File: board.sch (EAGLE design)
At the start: 75 parts, among them IC1 LM1117, J1 LHBEAMOUT, J10 ATEMP, J11 HORNOUT, J12 12V_SUPPLY, J13 STOPOUT, J14 TURNOUT, J15 FANOUT, J16 BLIGHTOUT, J17 AUXOUT, J18 AUX, J19 CAN, J2 BATT, J3 BLIGHT, J4 LHBEAM, J5 LRTURN, J6 WARNING, J7 HORN, J8 BREAK, J9 ABREAK, Q1 IRF7465TR, Q2 IRF7465TR, Q3 IRF7465TR, Q4 IRLML9301TRPBF, Q5 IRLML9301TRPBF, Q6 IRF7424TRPBF, Q7 IRF7424TRPBF, Q8 IRF7424TRPBF, Q9 IRLML9301TRPBF, U1 VOM1271T, U2 VOM1271T, U3 VOM1271T, U4 MC14504BDR2G, U5 MAX3051ESA+T

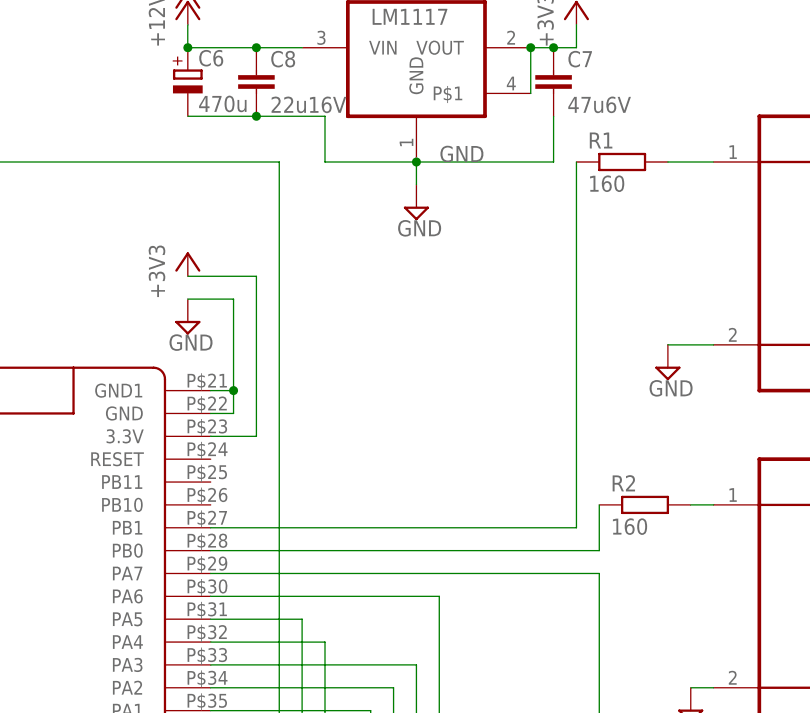
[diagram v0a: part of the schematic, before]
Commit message: Board & schematics v 1.1. Minor improvements
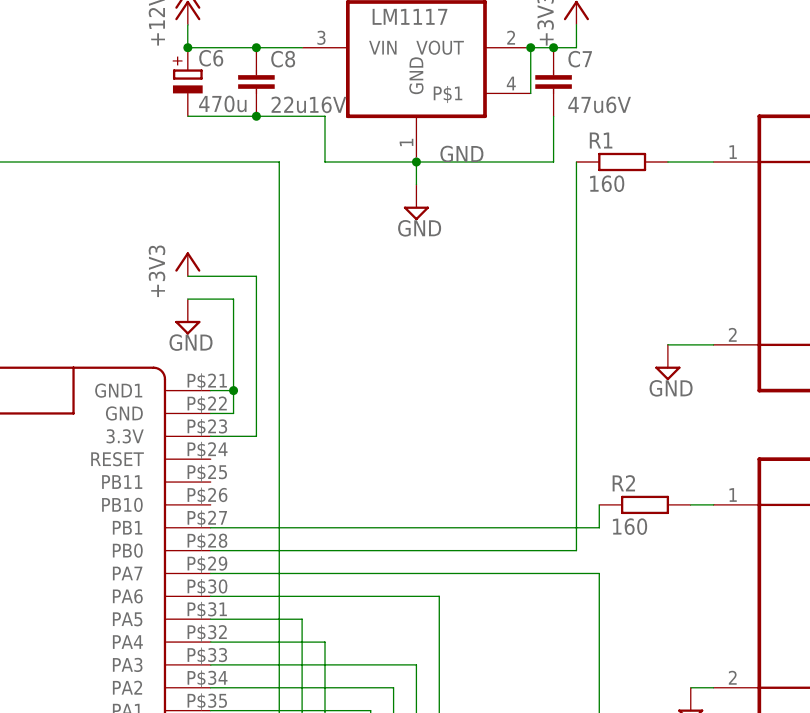
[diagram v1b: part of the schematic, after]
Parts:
- C2: device rcl:C-EUC0805 -> rcl:C-EUC1206
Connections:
- net N$1 renamed LVCTL4
- net N$13 renamed LVCTL2
- net N$14 renamed LVCTL3
- net N$2 renamed LVCTL5
- net N$20 renamed LV4G
- net N$24 renamed LV5G
- net N$25 renamed LV6G
- net N$26 renamed LV3G
- net N$27 renamed LV2G
- net N$28 renamed LV1G
- net N$3 renamed LVCTL6
- net N$37 renamed IATEMP
- net N$38 renamed ABRK
- net N$39 renamed ABRK_S
- net N$4 renamed HV1CTLG
- net N$5 renamed HV2CTLG
- net N$6 renamed HV3CTLG
- net N$7 renamed HV1G
- net N$8 renamed HV2G
- net N$9 renamed HV3G
- net HV1CTL: now also U$1.PB0; no longer U$1.PB1
- net HV2CTL: now also U$1.PB1; no longer U$1.PB0
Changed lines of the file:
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@@
 </spice>
 </part>
-<part name="C2" library="rcl" library_urn="urn:adsk.eagle:library:334" deviceset="C-EU" device="C0805" package3d_urn="urn:adsk.eagle:package:23617/2" value="0.1u"/>
+<part name="C2" library="rcl" library_urn="urn:adsk.eagle:library:334" deviceset="C-EU" device="C1206" package3d_urn="urn:adsk.eagle:package:23618/2" value="0.1u"/>
 <part name="C3" library="rcl" library_urn="urn:adsk.eagle:library:334" deviceset="C-EU" device="C0805" package3d_urn="urn:adsk.eagle:package:23617/2" value="0.1u"/>
 <part name="LOGO2" library="SparkFun-Aesthetics" deviceset="OSHW-LOGO" device="L"/>
@@
 <net name="HV1CTL" class="0">
 <segment>
+<pinref part="R1" gate="G$1" pin="1"/>
+<wire x1="-20.32" y1="114.3" x2="-20.32" y2="157.48" width="0.1524" layer="91"/>
+<pinref part="U$1" gate="G$1" pin="PB0"/>
+<wire x1="-20.32" y1="114.3" x2="-60.96" y2="114.3" width="0.1524" layer="91"/>
+</segment>
+</net>
+<net name="HV2CTL" class="0">
+<segment>
+<pinref part="R2" gate="G$1" pin="1"/>
 <pinref part="U$1" gate="G$1" pin="PB1"/>
-<wire x1="-60.96" y1="116.84" x2="-20.32" y2="116.84" width="0.1524" layer="91"/>
-<pinref part="R1" gate="G$1" pin="1"/>
-<wire x1="-20.32" y1="116.84" x2="-20.32" y2="157.48" width="0.1524" layer="91"/>
-</segment>
-</net>
-<net name="HV2CTL" class="0">
-<segment>
-<pinref part="U$1" gate="G$1" pin="PB0"/>
-<wire x1="-60.96" y1="114.3" x2="-17.78" y2="114.3" width="0.1524" layer="91"/>
-<wire x1="-17.78" y1="114.3" x2="-17.78" y2="119.38" width="0.1524" layer="91"/>
-<pinref part="R2" gate="G$1" pin="1"/>
+<wire x1="-17.78" y1="116.84" x2="-17.78" y2="119.38" width="0.1524" layer="91"/>
+<wire x1="-60.96" y1="116.84" x2="-17.78" y2="116.84" width="0.1524" layer="91"/>
 </segment>
 </net>
@@
 </segment>
 </net>
-<net name="N$5" class="0">
+<net name="HV2CTLG" class="0">
 <segment>
 <pinref part="U2" gate="G$1" pin="A1"/>
@@
 </segment>
 </net>
-<net name="N$6" class="0">
+<net name="HV3CTLG" class="0">
 <segment>
 <pinref part="U3" gate="G$1" pin="A1"/>
@@
 </segment>
 </net>
-<net name="N$4" class="0">
+<net name="HV1CTLG" class="0">
 <segment>
 <pinref part="R1" gate="G$1" pin="2"/>
@@
 </segment>
 </net>
-<net name="N$7" class="0">
+<net name="HV1G" class="0">
 <segment>
 <pinref part="U1" gate="G$1" pin="A2"/>
@@
 </segment>
 </net>
-<net name="N$8" class="0">
+<net name="HV2G" class="0">
 <segment>
 <pinref part="U2" gate="G$1" pin="A2"/>
@@
 </segment>
 </net>
-<net name="N$9" class="0">
+<net name="HV3G" class="0">
 <segment>
 <pinref part="U3" gate="G$1" pin="A2"/>
@@
 </segment>
 </net>
-<net name="N$1" class="0">
+<net name="LVCTL4" class="0">
 <segment>
 <pinref part="U$1" gate="G$1" pin="PA3"/>
@@
 </segment>
 </net>
-<net name="N$2" class="0">
+<net name="LVCTL5" class="0">
 <segment>
 <pinref part="U$1" gate="G$1" pin="PA2"/>
@@
 </segment>
 </net>
-<net name="N$3" class="0">
+<net name="LVCTL6" class="0">
 <segment>
 <pinref part="U$1" gate="G$1" pin="PA1"/>
@@
 </segment>
 </net>
-<net name="N$13" class="0">
+<net name="LVCTL2" class="0">
 <segment>
 <pinref part="U$1" gate="G$1" pin="PB7"/>
@@
 </segment>
 </net>
-<net name="N$14" class="0">
+<net name="LVCTL3" class="0">
 <segment>
 <pinref part="U$1" gate="G$1" pin="PB6"/>
@@
 </segment>
 </net>
-<net name="N$20" class="0">
+<net name="LV4G" class="0">
 <segment>
 <pinref part="U4" gate="A" pin="AOUT"/>
@@
 </segment>
 </net>
-<net name="N$24" class="0">
+<net name="LV5G" class="0">
 <segment>
 <pinref part="U4" gate="A" pin="BOUT"/>
@@
 </segment>
 </net>
-<net name="N$25" class="0">
+<net name="LV6G" class="0">
 <segment>
 <pinref part="U4" gate="A" pin="COUT"/>
@@
 </segment>
 </net>
-<net name="N$26" class="0">
+<net name="LV3G" class="0">
 <segment>
 <pinref part="Q6" gate="G$1" pin="G"/>
@@
 </segment>
 </net>
-<net name="N$27" class="0">
+<net name="LV2G" class="0">
 <segment>
 <wire x1="-27.94" y1="48.26" x2="-27.94" y2="-35.56" width="0.1524" layer="91"/>
@@
 </segment>
 </net>
-<net name="N$28" class="0">
+<net name="LV1G" class="0">
 <segment>
 <pinref part="U4" gate="A" pin="FOUT"/>
@@
 </segment>
 </net>
-<net name="N$37" class="0">
+<net name="IATEMP" class="0">
 <segment>
 <pinref part="J10" gate="G$1" pin="2"/>
@@
 </segment>
 </net>
-<net name="N$38" class="0">
+<net name="ABRK" class="0">
 <segment>
 <pinref part="J9" gate="G$1" pin="2"/>
@@
 </segment>
 </net>
-<net name="N$39" class="0">
+<net name="ABRK_S" class="0">
 <segment>
 <pinref part="R13" gate="G$1" pin="2"/>

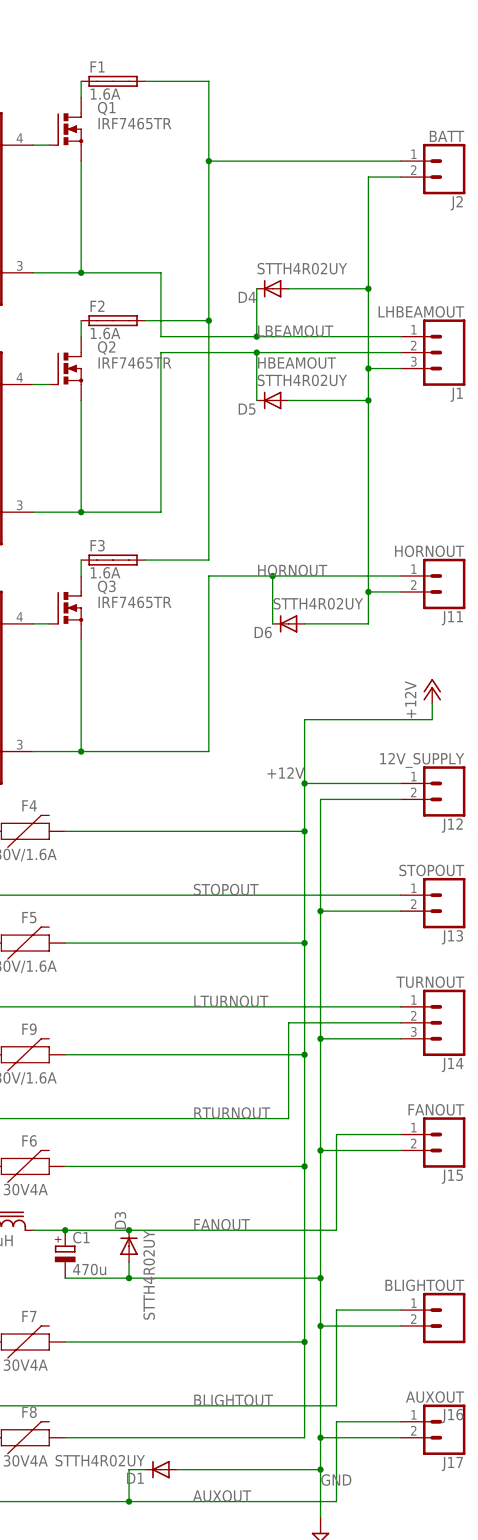
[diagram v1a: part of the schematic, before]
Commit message: Added BOM
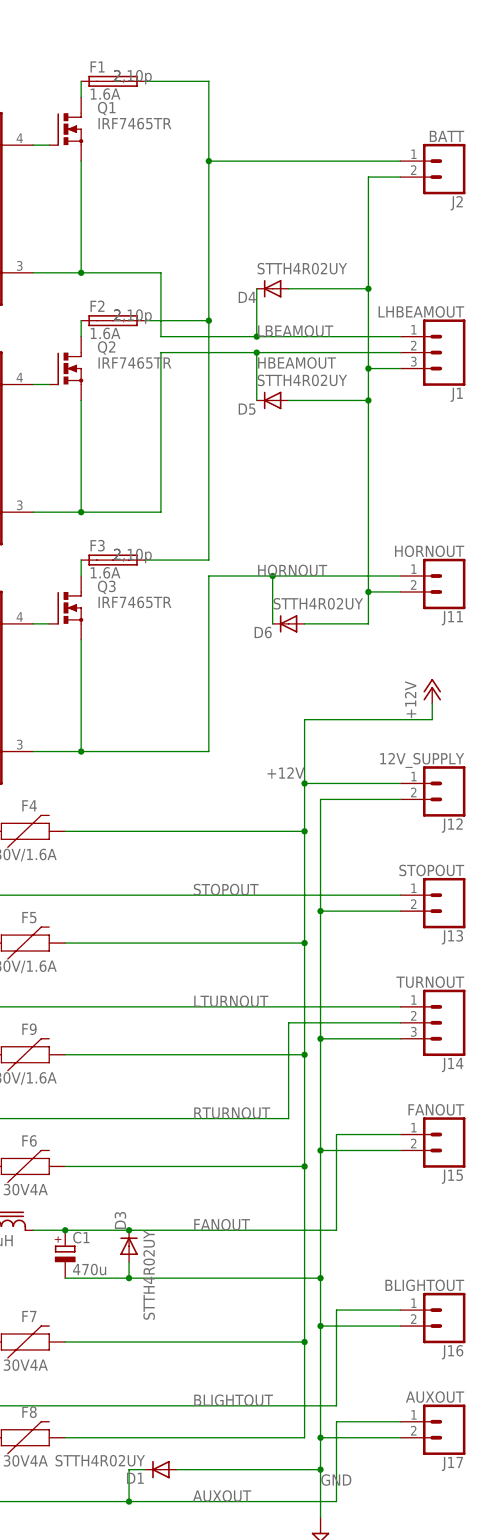
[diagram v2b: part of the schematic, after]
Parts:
- C1, C6: MPN (none) -> SK016M0470B3F-0811; PRICE (none) -> 2,70р; SHOP (none) -> https://www.terraelectronica.ru/product/1262453
- C2: MPN (none) -> CC1206KRX7R8BB104; PRICE (none) -> 2,20р; SHOP (none) -> https://www.terraelectronica.ru/product/540763
- C3: MPN (none) -> CC0805KRX7R9BB104; PRICE (none) -> 2,00р; SHOP (none) -> https://www.terraelectronica.ru/product/251110
- C7: MPN CL31A476MQHNNNE -> CL31A476MQHNNNE; PRICE (none) -> 7,70р; SHOP (none) -> https://www.terraelectronica.ru/product/882710
- C8: MPN CL32A226KOJNNNE -> CL31A226KOHNNNE; PRICE (none) -> 12,80р; SHOP (none) -> https://www.terraelectronica.ru/product/1641407
- D1, D3, D4, D5, D6: MPN STTH4R02UY -> STTH4R02U; PRICE (none) -> 14,10р; SHOP (none) -> https://www.terraelectronica.ru/product/450947
- F1, F2, F3: MPN (none) -> FC-001S; PRICE (none) -> 2,10р; QTY (none) -> 2; SHOP (none) -> https://www.terraelectronica.ru/product/2076693
- F4, F5, F9: PRICE (none) -> 5,40р; SHOP (none) -> https://www.terraelectronica.ru/product/1040513
- F6, F7, F8: PRICE (none) -> 25,90р; SHOP (none) -> https://www.terraelectronica.ru/product/577123
- IC1: MPN (none) -> LD1117S33TR; PRICE (none) -> 12,00р; SHOP (none) -> https://www.terraelectronica.ru/product/208059
- J1, J14, J4, J5: MPN (none) -> DG350-3.5-03P-14-00AH; PRICE (none) -> 9,40р; SHOP (none) -> https://www.terraelectronica.ru/product/1108750
- J10, J11, J12, J13, J15, J16, J17, J18, J19, J2, J3, J6, J7, J8, J9: MPN (none) -> DG350-3.5-02P-14-00AH; PRICE (none) -> 5,80р; SHOP (none) -> https://www.terraelectronica.ru/product/1115132
- L1: MPN (none) -> SDR1307-150ML; PRICE (none) -> 21,20р; SHOP (none) -> https://www.terraelectronica.ru/product/607745
- Q1, Q2, Q3: MPN (none) -> IRF7465TRPBF; PRICE (none) -> 26,30р; SHOP (none) -> https://www.terraelectronica.ru/product/507651
- Q4, Q5, Q9: MPN (none) -> IRLML9301TRPBF; PRICE (none) -> 9,10р; SHOP (none) -> https://www.terraelectronica.ru/product/575910
- Q6, Q7, Q8: MPN (none) -> IRF7424TRPBF; PRICE (none) -> 15,40р; SHOP (none) -> https://www.terraelectronica.ru/product/301875
- R1: PRICE (none) -> 0,52р; SHOP (none) -> https://www.terraelectronica.ru/product/880371
- R13: MPN (none) -> RC0805JR-071KL; PRICE (none) -> 0,17р; SHOP (none) -> https://www.terraelectronica.ru/product/443003
- R14: MPN (none) -> RC0805FR-072K4L; PRICE (none) -> 0,15р; SHOP (none) -> https://www.terraelectronica.ru/product/562267
- R15: MPN (none) -> RC0805JR-0710KL; PRICE (none) -> 0,24р; SHOP (none) -> https://www.terraelectronica.ru/product/339147
- R16: MPN (none) -> RC0805FR-07120RL; PRICE (none) -> 0,23р; SHOP (none) -> https://www.terraelectronica.ru/product/542987
- R4: MPN (none) -> RC0805JR-071KL; PRICE (none) -> 0,19р; SHOP (none) -> https://www.terraelectronica.ru/product/559515
- U$1: MPN (none) -> Blue Pill; PRICE (none) -> 127,73р; SHOP (none) -> https://ru.aliexpress.com/item/STM32F103C8T6-ARM-STM32-Mini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
- U1, U2, U3: MPN (none) -> VOM1271T; PRICE (none) -> 173,00р; SHOP (none) -> https://www.terraelectronica.ru/product/1112827
- U4: MPN (none) -> MC14504BDR2G; PRICE (none) -> 25,70р; SHOP (none) -> https://www.terraelectronica.ru/product/284776
- U5: MPN (none) -> MAX3051ESA+T; PRICE (none) -> 141,00р; SHOP (none) -> https://www.terraelectronica.ru/product/462120
